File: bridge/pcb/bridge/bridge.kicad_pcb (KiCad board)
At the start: 2 copper layers, 163 x 83 mm, 28 parts, among them J1 Screw_Terminal_01x06, J2 Screw_Terminal_01x06, J3 Screw_Terminal_01x06, J4 Conn_01x23, Q1 PMOS, Q2 PMOS, Q3 PMOS, Q4 PMOS, Q5 PMOS, SW1 SW_SPST, U1 YAAJ_BluePill, U2 J104D2C12VDC.20S, U3 AD557JN

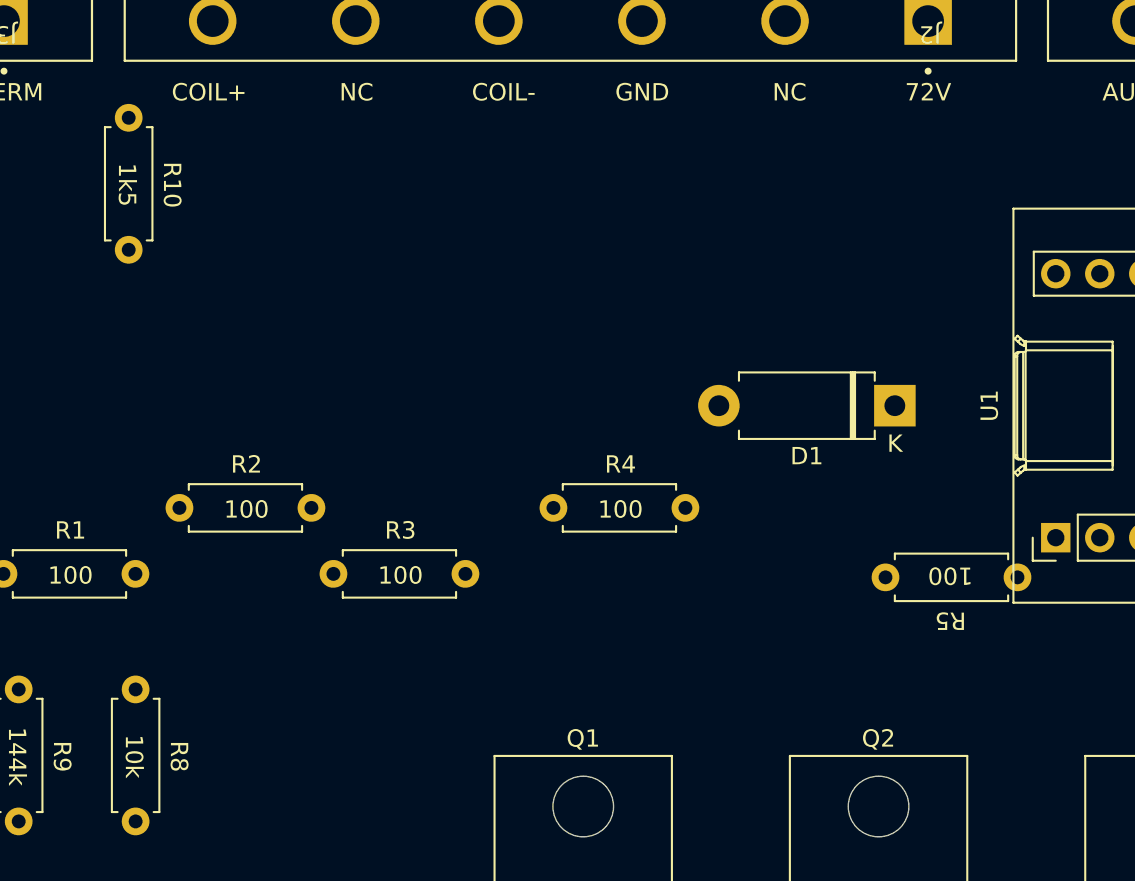
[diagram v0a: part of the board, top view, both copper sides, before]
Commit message: Completed schematic
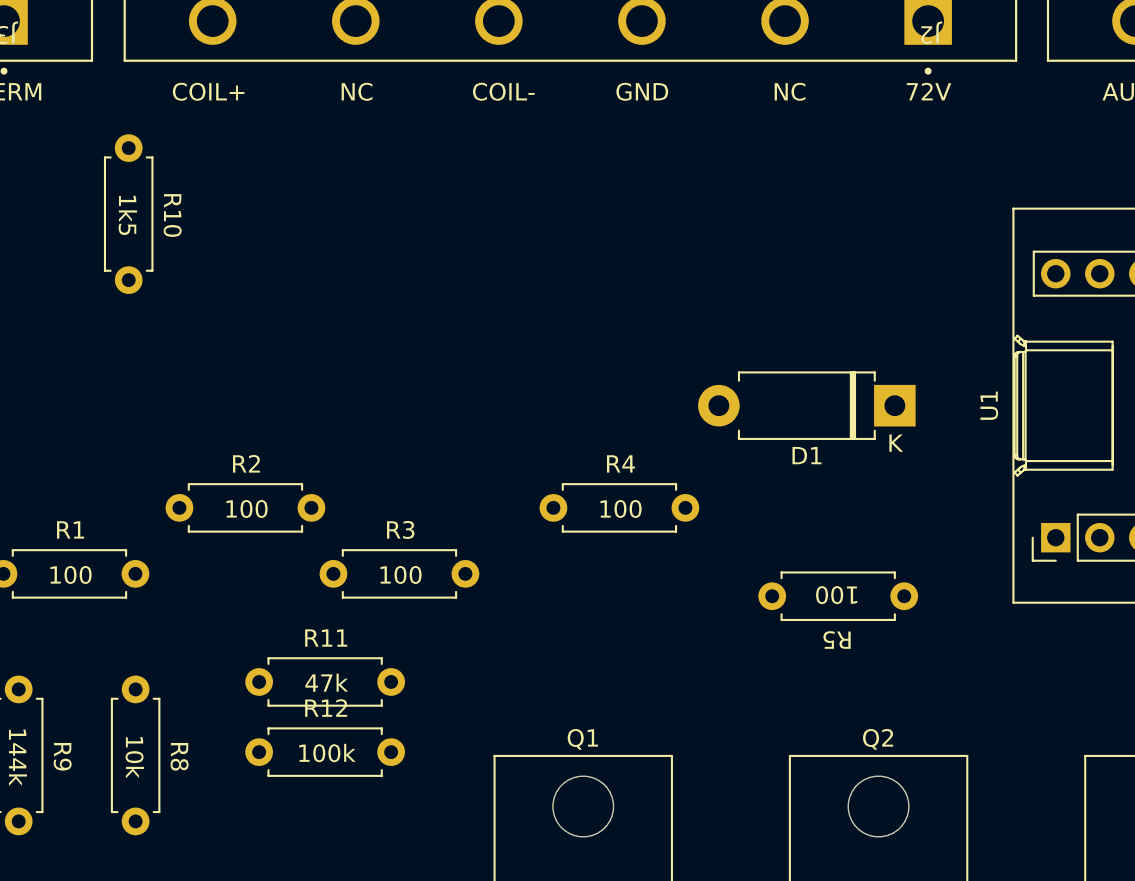
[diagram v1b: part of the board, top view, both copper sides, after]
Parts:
- added R11: 47k, bridge:THT_RESISTOR_WITH_VALUE, F.Cu at (129.2, 92.0)
- added R12: 100k, bridge:THT_RESISTOR_WITH_VALUE, F.Cu at (129.2, 96.1)
- moved R5 6.63 mm to (158.8, 86.9)
- moved R10 1.75 mm to (117.8, 65.0)
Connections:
- U1 pad 11: unconnected-(U1-PB3-Pad11) -> MAN_AUTO_STATE
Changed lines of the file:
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@@
   (net 49 "unconnected-(U1-PA12-Pad9)")
   (net 50 "unconnected-(U1-PA15-Pad10)")
-  (net 51 "unconnected-(U1-PB3-Pad11)")
+  (net 51 "MAN_AUTO_STATE")
   (net 52 "unconnected-(U1-3V3-Pad20)")
   (net 53 "unconnected-(U1-VBat-Pad21)")
@@
     )
   )
+  (footprint "bridge:THT_RESISTOR_WITH_VALUE" (layer "F.Cu")
+    (at 129.25 96.1)
+    (property "Sheetfile" "bridge.kicad_sch")
+    (property "Sheetname" "")
+    (property "ki_description" "Resistor")
+    (property "ki_keywords" "R res resistor")
+    (attr through_hole)
+    (fp_text reference "R12" (at 0 -2.6 unlocked) (layer "F.SilkS")
+        (effects (font (size 1 1) (thickness 0.1)))
+    )
+    (fp_text value "100k" (at 0 0 unlocked) (layer "F.SilkS")
+        (effects (font (size 1 1) (thickness 0.15)))
+    )
+    (fp_text user "${REFERENCE}" (at 0 2.5 unlocked) (layer "F.Fab")
+        (effects (font (size 1 1) (thickness 0.15)))
+    )
+    (fp_line (start -3.33 -1.47) (end 3.21 -1.47)
+      (stroke (width 0.12) (type solid)) (layer "F.SilkS"))
+    (fp_line (start -3.33 -1.14) (end -3.33 -1.47)
+      (stroke (width 0.12) (type solid)) (layer "F.SilkS"))
+    (fp_line (start -3.33 0.94) (end -3.33 1.27)
+      (stroke (width 0.12) (type solid)) (layer "F.SilkS"))
+    (fp_line (start -3.33 1.27) (end 3.21 1.27)
+      (stroke (width 0.12) (type solid)) (layer "F.SilkS"))
+    (fp_line (start 3.21 -1.47) (end 3.21 -1.14)
+      (stroke (width 0.12) (type solid)) (layer "F.SilkS"))
+    (fp_line (start 3.21 1.27) (end 3.21 0.94)
+      (stroke (width 0.12) (type solid)) (layer "F.SilkS"))
+    (fp_line (start -4.92 -1.6) (end -4.92 1.4)
+      (stroke (width 0.05) (type solid)) (layer "F.CrtYd"))
+    (fp_line (start -4.92 1.4) (end 4.8 1.4)
+      (stroke (width 0.05) (type solid)) (layer "F.CrtYd"))
+    (fp_line (start 4.8 -1.6) (end -4.92 -1.6)
+      (stroke (width 0.05) (type solid)) (layer "F.CrtYd"))
+    (fp_line (start 4.8 1.4) (end 4.8 -1.6)
+      (stroke (width 0.05) (type solid)) (layer "F.CrtYd"))
+    (fp_line (start -3.87 -0.1) (end -3.21 -0.1)
+      (stroke (width 0.1) (type solid)) (layer "F.Fab"))
+    (fp_line (start -3.21 -1.35) (end -3.21 1.15)
+      (stroke (width 0.1) (type solid)) (layer "F.Fab"))
+    (fp_line (start -3.21 1.15) (end 3.09 1.15)
+      (stroke (width 0.1) (type solid)) (layer "F.Fab"))
+    (fp_line (start 3.09 -1.35) (end -3.21 -1.35)
+      (stroke (width 0.1) (type solid)) (layer "F.Fab"))
+    (fp_line (start 3.09 1.15) (end 3.09 -1.35)
+      (stroke (width 0.1) (type solid)) (layer "F.Fab"))
+    (fp_line (start 3.75 -0.1) (end 3.09 -0.1)
+      (stroke (width 0.1) (type solid)) (layer "F.Fab"))
+    (pad "1" thru_hole circle (at -3.87 -0.1) (size 1.6 1.6) (drill 0.8) (layers "*.Cu" "*.Mask")
+      (net 51 "MAN_AUTO_STATE") (pintype "passive"))
+    (pad "2" thru_hole oval (at 3.75 -0.1) (size 1.6 1.6) (drill 0.8) (layers "*.Cu" "*.Mask")
+      (net 73 "Net-(SW1-A)") (pintype "passive"))
+    (model "${KICAD6_3DMODEL_DIR}/Resistor_THT.3dshapes/R_Axial_DIN0207_L6.3mm_D2.5mm_P7.62mm_Horizontal.wrl"
+      (offset (xyz -4 0 0))
+      (scale (xyz 1 1 1))
+      (rotate (xyz 0 0 0))
+    )
+  )
   (footprint "Package_TO_SOT_THT:TO-220-3_Horizontal_TabDown" (layer "F.Cu")
     (at 141.55 115.8)
@@
   )
   (footprint "bridge:THT_RESISTOR_WITH_VALUE" (layer "F.Cu")
-    (at 165.29 85.81 180)
+    (at 158.75 86.9 180)
     (property "Sheetfile" "mcu.kicad_sch")
     (property "Sheetname" "MCU")
@@
   )
   (footprint "bridge:THT_RESISTOR_WITH_VALUE" (layer "F.Cu")
-    (at 117.75 63.25 -90)
+    (at 117.75 65 -90)
     (property "Sheetfile" "mcu.kicad_sch")
     (property "Sheetname" "MCU")
@@
   )
   (footprint "bridge:THT_RESISTOR_WITH_VALUE" (layer "F.Cu")
+    (at 129.25 92.05)
+    (property "Sheetfile" "bridge.kicad_sch")
+    (property "Sheetname" "")
+    (property "ki_description" "Resistor")
+    (property "ki_keywords" "R res resistor")
+    (attr through_hole)
+    (fp_text reference "R11" (at 0 -2.6 unlocked) (layer "F.SilkS")
+        (effects (font (size 1 1) (thickness 0.1)))
+    )
+    (fp_text value "47k" (at 0 0 unlocked) (layer "F.SilkS")
+        (effects (font (size 1 1) (thickness 0.15)))
+    )
+    (fp_text user "${REFERENCE}" (at 0 2.5 unlocked) (layer "F.Fab")
+        (effects (font (size 1 1) (thickness 0.15)))
+    )
+    (fp_line (start -3.33 -1.47) (end 3.21 -1.47)
+      (stroke (width 0.12) (type solid)) (layer "F.SilkS"))
+    (fp_line (start -3.33 -1.14) (end -3.33 -1.47)
+      (stroke (width 0.12) (type solid)) (layer "F.SilkS"))
+    (fp_line (start -3.33 0.94) (end -3.33 1.27)
+      (stroke (width 0.12) (type solid)) (layer "F.SilkS"))
+    (fp_line (start -3.33 1.27) (end 3.21 1.27)
+      (stroke (width 0.12) (type solid)) (layer "F.SilkS"))
+    (fp_line (start 3.21 -1.47) (end 3.21 -1.14)
+      (stroke (width 0.12) (type solid)) (layer "F.SilkS"))
+    (fp_line (start 3.21 1.27) (end 3.21 0.94)
+      (stroke (width 0.12) (type solid)) (layer "F.SilkS"))
+    (fp_line (start -4.92 -1.6) (end -4.92 1.4)
+      (stroke (width 0.05) (type solid)) (layer "F.CrtYd"))
+    (fp_line (start -4.92 1.4) (end 4.8 1.4)
+      (stroke (width 0.05) (type solid)) (layer "F.CrtYd"))
+    (fp_line (start 4.8 -1.6) (end -4.92 -1.6)
+      (stroke (width 0.05) (type solid)) (layer "F.CrtYd"))
+    (fp_line (start 4.8 1.4) (end 4.8 -1.6)
+      (stroke (width 0.05) (type solid)) (layer "F.CrtYd"))
+    (fp_line (start -3.87 -0.1) (end -3.21 -0.1)
+      (stroke (width 0.1) (type solid)) (layer "F.Fab"))
+    (fp_line (start -3.21 -1.35) (end -3.21 1.15)
+      (stroke (width 0.1) (type solid)) (layer "F.Fab"))
+    (fp_line (start -3.21 1.15) (end 3.09 1.15)
+      (stroke (width 0.1) (type solid)) (layer "F.Fab"))
+    (fp_line (start 3.09 -1.35) (end -3.21 -1.35)
+      (stroke (width 0.1) (type solid)) (layer "F.Fab"))
+    (fp_line (start 3.09 1.15) (end 3.09 -1.35)
+      (stroke (width 0.1) (type solid)) (layer "F.Fab"))
+    (fp_line (start 3.75 -0.1) (end 3.09 -0.1)
+      (stroke (width 0.1) (type solid)) (layer "F.Fab"))
+    (pad "1" thru_hole circle (at -3.87 -0.1) (size 1.6 1.6) (drill 0.8) (layers "*.Cu" "*.Mask")
+      (net 5 "GND") (pintype "passive"))
+    (pad "2" thru_hole oval (at 3.75 -0.1) (size 1.6 1.6) (drill 0.8) (layers "*.Cu" "*.Mask")
+      (net 51 "MAN_AUTO_STATE") (pintype "passive"))
+    (model "${KICAD6_3DMODEL_DIR}/Resistor_THT.3dshapes/R_Axial_DIN0207_L6.3mm_D2.5mm_P7.62mm_Horizontal.wrl"
+      (offset (xyz -4 0 0))
+      (scale (xyz 1 1 1))
+      (rotate (xyz 0 0 0))
+    )
+  )
+  (footprint "bridge:THT_RESISTOR_WITH_VALUE" (layer "F.Cu")
     (at 146.24 82)
     (property "Sheetfile" "mcu.kicad_sch")
@@
       (net 50 "unconnected-(U1-PA15-Pad10)") (pinfunction "PA15") (pintype "bidirectional+no_connect"))
     (pad "11" thru_hole circle (at 0 25.4 90) (size 1.7 1.7) (drill 1) (layers "*.Cu" "*.Mask")
-      (net 51 "unconnected-(U1-PB3-Pad11)") (pinfunction "PB3") (pintype "bidirectional+no_connect"))
+      (net 51 "MAN_AUTO_STATE") (pinfunction "PB3") (pintype "bidirectional"))
     (pad "12" thru_hole circle (at 0 27.94 90) (size 1.7 1.7) (drill 1) (layers "*.Cu" "*.Mask")
       (net 4 "START_SWITCH_NEG_MAN") (pinfunction "PB4") (pintype "bidirectional"))
